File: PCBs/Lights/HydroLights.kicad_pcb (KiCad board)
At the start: 2 copper layers, 135.6 x 17.3 mm, 15 parts, among them U1 Solder_Pad, U10 Solder_Pad, U11 Solder_Pad, U2 Solder_Pad, U3 158303250A_(Daylight), U4 150283HS73103 (Red) 2.2v 150mA, U5 158303250A_(Daylight), U6 150283BS73103 (Blue) 3.2v 150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, U7 158303250A_(Daylight), U8 150283GS73103 (Green) 3v 150mA, U9 158303250A_(Daylight)

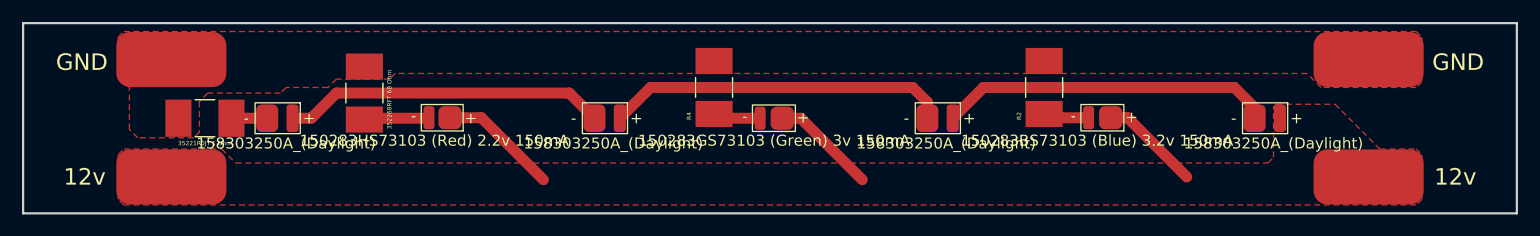
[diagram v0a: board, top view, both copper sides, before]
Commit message: Finished PCBs
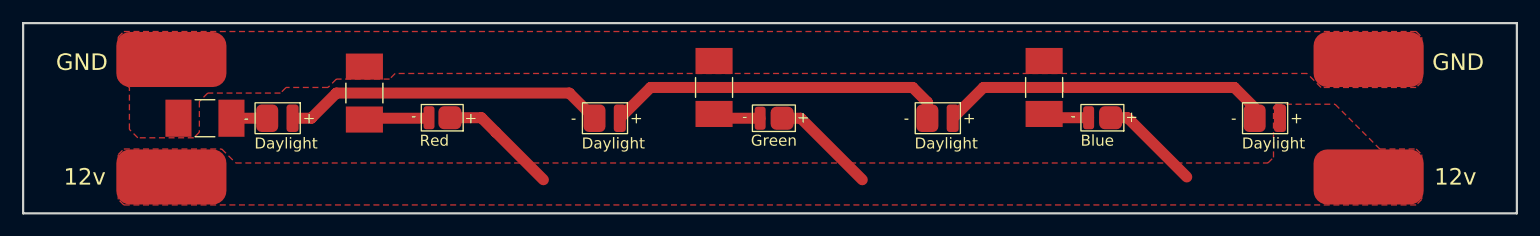
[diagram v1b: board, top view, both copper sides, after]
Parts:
- U3, U5, U7, U9: value 158303250A_(Daylight) -> Daylight
- U4: value 150283HS73103 (Red) 2.2v 150mA -> Red
- U6: value 150283BS73103 (Blue) 3.2v 150mA -> Blue
- U8: value 150283GS73103 (Green) 3v 150mA -> Green
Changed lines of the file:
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@@
     (pad_to_mask_clearance 0)
     (pcbplotparams
-      (layerselection 0x00010fc_ffffffff)
+      (layerselection 0x00010f0_ffffffff)
       (disableapertmacros false)
       (usegerberextensions false)
-      (usegerberattributes true)
+      (usegerberattributes false)
       (usegerberadvancedattributes true)
       (creategerberjobfile true)
@@
       (effects (font (size 1 1) (thickness 0.15)))
     )
-    (fp_text value "158303250A_(Daylight)" (at 0.762 2.286 unlocked) (layer "F.SilkS")
+    (fp_text value "Daylight" (at 0.762 2.286 unlocked) (layer "F.SilkS")
       (effects (font (size 1 1) (thickness 0.15)))
     )
@@
       (effects (font (size 1 1) (thickness 0.15)))
     )
-    (fp_text value "158303250A_(Daylight)" (at 0.762 2.286 unlocked) (layer "F.SilkS")
+    (fp_text value "Daylight" (at 0.762 2.286 unlocked) (layer "F.SilkS")
       (effects (font (size 1 1) (thickness 0.15)))
     )
@@
       (effects (font (size 1 1) (thickness 0.15)))
     )
-    (fp_text value "158303250A_(Daylight)" (at 0.762 2.286 unlocked) (layer "F.SilkS")
+    (fp_text value "Daylight" (at 0.762 2.286 unlocked) (layer "F.SilkS")
       (effects (font (size 1 1) (thickness 0.15)))
     )
@@
       (effects (font (size 1 1) (thickness 0.15)))
     )
-    (fp_text value "158303250A_(Daylight)" (at 0.762 2.286 unlocked) (layer "F.SilkS")
+    (fp_text value "Daylight" (at 0.762 2.286 unlocked) (layer "F.SilkS")
       (effects (font (size 1 1) (thickness 0.15)))
     )
@@
       (effects (font (size 0.393701 0.393701) (thickness 0.15)))
     )
-    (fp_text value "352268RFT 68 Ohm" (at -0.59 2.27 90) (layer "F.SilkS")
+    (fp_text value "352268RFT 68 Ohm" (at -0.59 2.27 90) (layer "F.SilkS") hide
       (effects (font (size 0.393701 0.393701) (thickness 0.15)))
     )
@@
       (effects (font (size 1 1) (thickness 0.15)))
     )
-    (fp_text value "150283BS73103 (Blue) 3.2v 150mA" (at 2.313 -0.977 unlocked) (layer "F.SilkS")
+    (fp_text value "Blue" (at 2.313 -0.977 unlocked) (layer "F.SilkS")
       (effects (font (size 1 1) (thickness 0.15)))
     )
@@
       (effects (font (size 1 1) (thickness 0.15)))
     )
-    (fp_text value "150283GS73103 (Green) 3v 150mA" (at -0.1 -2.032 unlocked) (layer "F.SilkS")
+    (fp_text value "Green" (at -0.1 -2.032 unlocked) (layer "F.SilkS")
       (effects (font (size 1 1) (thickness 0.15)))
     )
@@
       (effects (font (size 0.393701 0.393701) (thickness 0.15)))
     )
-    (fp_text value "35221R0JT 1 Ohm" (at 0 2.27) (layer "F.SilkS")
+    (fp_text value "35221R0JT 1 Ohm" (at 0 2.27) (layer "F.SilkS") hide
       (effects (font (size 0.393701 0.393701) (thickness 0.15)))
     )
@@
       (effects (font (size 1 1) (thickness 0.15)))
     )
-    (fp_text value "150283HS73103 (Red) 2.2v 150mA" (at 2.517 -0.977 unlocked) (layer "F.SilkS")
+    (fp_text value "Red" (at 2.517 -0.977 unlocked) (layer "F.SilkS")
       (effects (font (size 1 1) (thickness 0.15)))
     )
@@
     (property "Sheetname" "")
     (attr smd)
-    (fp_text reference "R4" (at -2.59 -2.27 90) (layer "F.SilkS")
-      (effects (font (size 0.393701 0.393701) (thickness 0.15)))
-    )
-    (fp_text value "352262RFT 62 Ohm" (at -0.59 2.27 90) (layer "F.Fab")
+    (fp_text reference "R4" (at -2.59 -2.27 90) (layer "F.SilkS") hide
+      (effects (font (size 0.393701 0.393701) (thickness 0.15)))
+    )
+    (fp_text value "352262RFT 62 Ohm" (at -0.59 2.27 90) (layer "F.Fab") hide
       (effects (font (size 0.393701 0.393701) (thickness 0.15)))
     )
@@
     (property "Sheetname" "")
     (attr smd)
-    (fp_text reference "R2" (at -2.59 -2.27 90) (layer "F.SilkS")
-      (effects (font (size 0.393701 0.393701) (thickness 0.15)))
-    )
-    (fp_text value "352262RFT 62 Ohm" (at -0.59 2.27 90) (layer "F.Fab")
+    (fp_text reference "R2" (at -2.59 -2.27 90) (layer "F.SilkS") hide
+      (effects (font (size 0.393701 0.393701) (thickness 0.15)))
+    )
+    (fp_text value "352262RFT 62 Ohm" (at -0.59 2.27 90) (layer "F.Fab") hide
       (effects (font (size 0.393701 0.393701) (thickness 0.15)))
     )
@@
       (net 1 "GND") (pintype "input"))
   )
-  (gr_rect (start 204.47 88.138) (end 69.342 104.902) (layer "F.Mask") (width 0.15) (fill solid))
   (gr_rect (start 69.088 87.884) (end 204.724 105.156) (layer "Edge.Cuts") (width 0.2) (fill none))
   (gr_text "GND" (at 74.422 91.44) (layer "F.SilkS")
